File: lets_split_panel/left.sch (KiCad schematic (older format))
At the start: 69 parts, among them J1 Speaker, J2 RST, J3 ISP, P1 WS2812>, P2 USB_OTG, P3 >WS2812, P4 Conn_01x04, SW1 MXALPS, SW10 MXALPS, SW11 MXALPS, SW12 MXALPS, SW13 MXALPS, SW14 MXALPS, SW15 MXALPS, SW16 MXALPS, SW17 MXALPS, SW18 MXALPS, SW19 MXALPS, SW2 MXALPS, SW20 MXALPS, SW21 MXALPS, SW22 MXALPS, SW23 MXALPS, SW24 MXALPS, SW3 MXALPS, SW4 MXALPS, SW5 MXALPS, SW6 MXALPS, SW7 MXALPS, SW8 MXALPS, SW9 MXALPS, U1 ATMega32U4, Y1 Crystal

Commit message: I love git. Saved PCB file, started panel work
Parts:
- JP1, JP2: symbol JUMPER -> Jumper
- P1, P3: symbol CONN_01X03 -> Conn_01x03
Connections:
- net labels added: wd2812-in, ~Reset
- net labels removed: WD2812-in, ~RESET
- wire segments 132 -> 219

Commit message: Finished panel
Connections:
- net labels added: Dd+, Dd-
- wire segments 219 -> 154

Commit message: Added test jig for panel
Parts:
- removed P1: WS2812>, Wirepads:SMD_PAD_1x03_Pitch2.54mm, symbol Conn_01x03
- added J7: WS2812>, Pin_Headers:Pin_Header_Straight_1x01_Pitch2.54mm, symbol conn:Conn_01x01
- C1, C2, C3, C4: symbol C_Small -> lets_split_panel-rescue:C_Small-RESCUE-lets_split_panel
- D1, D10, D11, D12, D13, D14, D15, D16, D17, D18, D19, D2, D20, D21, D22, D23, D24, D3, D4, D5, D6, D7, D8, D9: symbol D -> lets_split_panel-rescue:D-RESCUE-lets_split_panel
- J1, J2: symbol Conn_01x02 -> lets_split_panel-rescue:Conn_01x02-RESCUE-lets_split_panel
- J3: footprint Jlink:J-link-needle-6pin -> Pin_Headers:Pin_Header_Straight_2x03_Pitch2.54mm; symbol Conn_02x03_Odd_Even -> lets_split_panel-rescue:Conn_02x03_Odd_Even-RESCUE-lets_split_panel
- JP1, JP2: symbol Jumper -> lets_split_panel-rescue:Jumper-RESCUE-lets_split_panel
- P2: symbol USB_OTG-RESCUE-lets_split -> lets_split_panel-rescue:USB_OTG-RESCUE-lets_split-RESCUE-lets_split_panel
- P3: symbol Conn_01x03 -> lets_split_panel-rescue:Conn_01x03-RESCUE-lets_split_panel
- P4: symbol Conn_01x04 -> lets_split_panel-rescue:Conn_01x04-RESCUE-lets_split_panel
- R1, R2, R3, R4, R5, R6: symbol R_Small -> lets_split_panel-rescue:R_Small-RESCUE-lets_split_panel
- SW1, SW10, SW11, SW12, SW13, SW14, SW15, SW16, SW17, SW18, SW19, SW2, SW20, SW21, SW22, SW23, SW24, SW3, SW4, SW5, SW6, SW7, SW8, SW9: symbol MXALPS -> lets_split_panel-rescue:MXALPS-RESCUE-lets_split_panel
- U1: symbol ATMega32U4 -> lets_split_panel-rescue:ATMega32U4-RESCUE-lets_split_panel
- Y1: symbol Crystal -> lets_split_panel-rescue:Crystal-RESCUE-lets_split_panel
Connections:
- wire segments 154 -> 150

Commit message: Changed to use SOT-23 dual diodes for cost
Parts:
- removed D1, D10, D11, D12, D13, D14, D15, D16, D17, D18, D19, D2, D20, D21, D22, D23, D24, D3, D4, D5, D6, D7, D8, D9: D, SeeedOPL-Diode-2016:SOD-123, symbol lets_split_panel-rescue:D-RESCUE-lets_split_panel
- removed SW1, SW10, SW11, SW12, SW13, SW14, SW15, SW16, SW17, SW18, SW19, SW2, SW20, SW21, SW22, SW23, SW24, SW3, SW4, SW5, SW6, SW7, SW8, SW9: MXALPS, CherryMX:Kailh-socket, symbol lets_split_panel-rescue:MXALPS-RESCUE-lets_split_panel
- added D1, D10, D11, D12, D2, D3, D4, D5, D6, D7, D8, D9: D_x2_KCom_AAK, TO_SOT_Packages_SMD:SOT-23, symbol device:D_x2_KCom_AAK
- added SW1, SW10, SW11, SW12, SW13, SW14, SW15, SW16, SW17, SW18, SW19, SW2, SW20, SW21, SW22, SW23, SW24, SW3, SW4, SW5, SW6, SW7, SW8, SW9: Socket, CherryMX:Kailh-socket, symbol switches:SW_Push
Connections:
- wire segments 150 -> 138
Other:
- moved on the sheet: P4

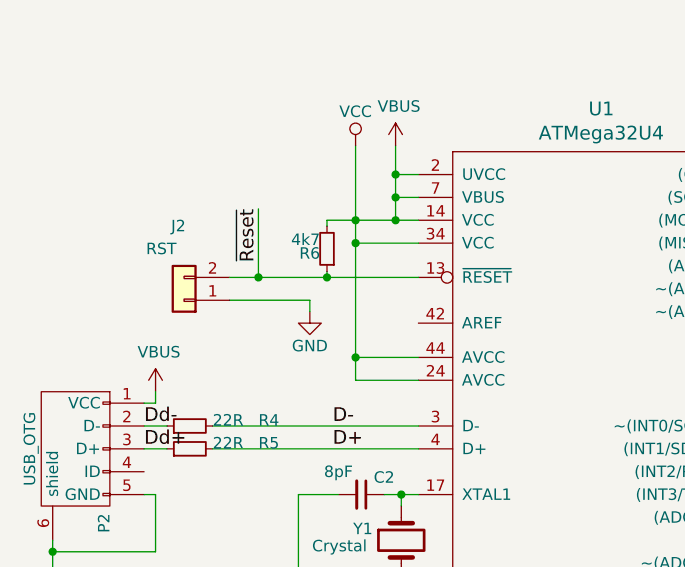
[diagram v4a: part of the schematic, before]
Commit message: Added fancy :)
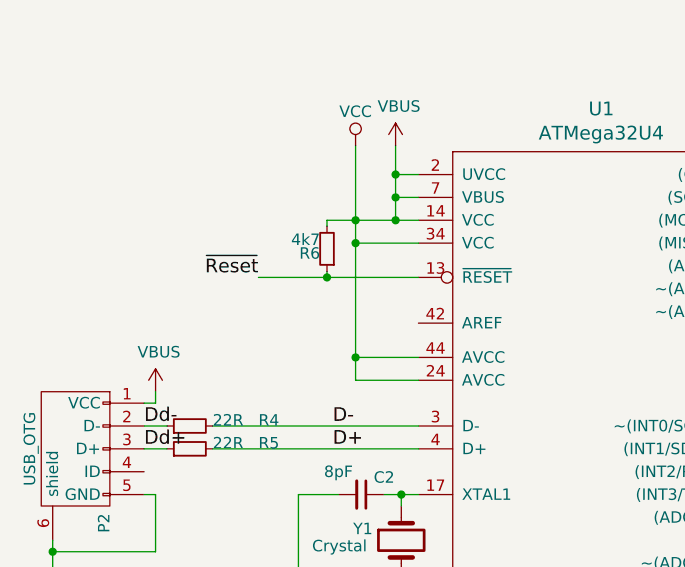
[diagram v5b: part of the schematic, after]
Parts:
- removed J2: RST, Pin_Headers:Pin_Header_Straight_1x02_Pitch2.54mm, symbol lets_split_panel-rescue:Conn_01x02-RESCUE-lets_split_panel
- C1, C4: footprint SeeedOPL-Capacitor-2016:C0603 -> Capacitors_SMD:C_0603
- C2, C3: footprint SeeedOPL-Capacitor-2016:C0402 -> Capacitors_SMD:C_0603
- R1, R2, R3, R4, R5, R6: footprint Resistors_SMD:R_0603_HandSoldering -> Resistors_SMD:R_0603
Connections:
- wire segments 138 -> 135
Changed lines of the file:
@@
 F 0 "R2" H 3530 2020 50  0000 L CNN
 F 1 "4k7" H 3530 1960 50  0000 L CNN
-F 2 "Resistors_SMD:R_0603_HandSoldering" H 3500 2000 50  0001 C CNN
+F 2 "Resistors_SMD:R_0603" H 3500 2000 50  0001 C CNN
 F 3 "" H 3500 2000 50  0000 C CNN
 	1    3500 2000
@@
 F 0 "R1" H 3430 2020 50  0000 L CNN
 F 1 "4k7" H 3430 1960 50  0000 L CNN
-F 2 "Resistors_SMD:R_0603_HandSoldering" H 3400 2000 50  0001 C CNN
+F 2 "Resistors_SMD:R_0603" H 3400 2000 50  0001 C CNN
 F 3 "" H 3400 2000 50  0000 C CNN
 	1    3400 2000
@@
 F 0 "R3" H 3305 3395 50  0000 L CNN
 F 1 "200" H 3305 3335 50  0000 L CNN
-F 2 "Resistors_SMD:R_0603_HandSoldering" H 3275 3375 50  0001 C CNN
+F 2 "Resistors_SMD:R_0603" H 3275 3375 50  0001 C CNN
 F 3 "" H 3275 3375 50  0000 C CNN
 	1    3275 3375
@@
 F 0 "R6" H 2230 4920 50  0000 L CNN
 F 1 "4k7" H 2230 4860 50  0000 L CNN
-F 2 "Resistors_SMD:R_0603_HandSoldering" H 2200 4900 50  0001 C CNN
+F 2 "Resistors_SMD:R_0603" H 2200 4900 50  0001 C CNN
 F 3 "" H 2200 4900 50  0000 C CNN
 	1    2200 4900
@@
 F 0 "C4" H 2542 6771 50  0000 L CNN
 F 1 "1uF" H 2542 6680 50  0000 L CNN
-F 2 "SeeedOPL-Capacitor-2016:C0603" H 2450 6725 50  0001 C CNN
+F 2 "Capacitors_SMD:C_0603" H 2450 6725 50  0001 C CNN
 F 3 "" H 2450 6725 50  0001 C CNN
 	1    2450 6725
@@
 F 0 "C2" V 2275 6075 50  0000 C CNN
 F 1 "8pF" V 2250 5875 50  0000 C CNN
-F 2 "SeeedOPL-Capacitor-2016:C0402" H 2350 5975 50  0001 C CNN
+F 2 "Capacitors_SMD:C_0603" H 2350 5975 50  0001 C CNN
 F 3 "" H 2350 5975 50  0001 C CNN
 	1    2350 5975
@@
 F 0 "C3" V 2525 6375 50  0000 C CNN
 F 1 "8pF" V 2450 6375 50  0000 C CNN
-F 2 "SeeedOPL-Capacitor-2016:C0402" H 2350 6375 50  0001 C CNN
+F 2 "Capacitors_SMD:C_0603" H 2350 6375 50  0001 C CNN
 F 3 "" H 2350 6375 50  0001 C CNN
 	1    2350 6375
@@
 F 0 "R4" V 1625 5375 50  0000 R CNN
 F 1 "22R" V 1625 5575 50  0000 R CNN
-F 2 "Resistors_SMD:R_0603_HandSoldering" H 1600 5675 50  0001 C CNN
+F 2 "Resistors_SMD:R_0603" H 1600 5675 50  0001 C CNN
 F 3 "" H 1600 5675 50  0000 C CNN
 	1    1600 5675
@@
 F 0 "R5" V 1625 5475 50  0000 R CNN
 F 1 "22R" V 1625 5675 50  0000 R CNN
-F 2 "Resistors_SMD:R_0603_HandSoldering" H 1600 5775 50  0001 C CNN
+F 2 "Resistors_SMD:R_0603" H 1600 5775 50  0001 C CNN
 F 3 "" H 1600 5775 50  0000 C CNN
 	1    1600 5775
@@
 F 0 "C1" H 2242 7321 50  0000 L CNN
 F 1 "1uF" H 2242 7230 50  0000 L CNN
-F 2 "SeeedOPL-Capacitor-2016:C0603" H 2150 7275 50  0001 C CNN
+F 2 "Capacitors_SMD:C_0603" H 2150 7275 50  0001 C CNN
 F 3 "" H 2150 7275 50  0001 C CNN
 	1    2150 7275
@@
 	-1   0    0    -1
 $EndComp
-$Comp
-L lets_split_panel-rescue:Conn_01x02-RESCUE-lets_split_panel J2
-U 1 1 5A0F48A9
-P 1575 5125
-F 0 "J2" H 1600 4800 50  0000 C CNN
-F 1 "RST" H 1675 4900 50  0000 C CNN
-F 2 "Pin_Headers:Pin_Header_Straight_1x02_Pitch2.54mm" H 1575 5125 50  0001 C CNN
-F 3 "" H 1575 5125 50  0001 C CNN
-	1    1575 5125
-	-1   0    0    1
-$EndComp
-$Comp
-L lets_split_panel-rescue:GND-RESCUE-lets_split_panel #PWR015
-U 1 1 5A0F501A
-P 2125 5175
-F 0 "#PWR015" H 2125 4925 50  0001 C CNN
-F 1 "GND" H 2125 5025 50  0000 C CNN
-F 2 "" H 2125 5175 50  0000 C CNN
-F 3 "" H 2125 5175 50  0000 C CNN
-	1    2125 5175
-	1    0    0    -1
-$EndComp
 Text Label 2225 5675 0    60   ~ 0
 D-
@@
 Wire Wire Line
 	6050 7050 6100 7050
-Connection ~ 1900 5025
-Wire Wire Line
-	1900 4725 1900 5025
 Connection ~ 3450 1225
 Wire Wire Line
@@
 Wire Wire Line
 	2600 6775 2550 6775
-Wire Wire Line
-	2125 5125 2125 5175
-Wire Wire Line
-	1775 5125 2125 5125
 Connection ~ 1000 6225
 Wire Wire Line
@@
 	2200 4775 2200 4800
 Connection ~ 2200 5025
-Wire Wire Line
-	1775 5025 2600 5025
 Wire Wire Line
 	2200 5025 2200 5000
@@
 Text Label 5500 7050 2    60   ~ 0
 ~Reset
-Text Label 1900 4725 3    60   ~ 0
+Text Label 1900 5025 2    60   ~ 0
 ~Reset
 Wire Wire Line
@@
 Connection ~ 10600 3525
 Connection ~ 10600 2875
+Wire Wire Line
+	1900 5025 2600 5025
 $EndSCHEMATC

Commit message: Seperated gerbers on request from board house
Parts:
- J7: symbol conn:Conn_01x01 -> lets_split_panel-rescue:Conn_01x01-RESCUE-lets_split_panel
- SW1, SW10, SW11, SW12, SW13, SW14, SW15, SW16, SW17, SW18, SW19, SW2, SW20, SW21, SW22, SW23, SW24, SW3, SW4, SW5, SW6, SW7, SW8, SW9: symbol switches:SW_Push -> lets_split_panel-rescue:SW_Push-RESCUE-lets_split_panel
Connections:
- wire segments 135 -> 182
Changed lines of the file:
@@
 	3500 1225 3500 1250
 Wire Wire Line
-	3400 1225 3500 1225
+	3400 1225 3450 1225
 Wire Wire Line
 	3400 1250 3400 1225
@@
 	1000 6225 1450 6225
 Wire Wire Line
-	2075 5975 2075 6450
+	2075 5975 2075 6375
 Wire Wire Line
 	2450 7275 2600 7275
@@
 	2075 5975 2250 5975
 Wire Wire Line
-	1000 6175 1000 6300
+	1000 6175 1000 6225
 Wire Wire Line
 	1450 5575 1450 5525
@@
 	2500 4675 2600 4675
 Wire Wire Line
-	2500 4775 2500 4450
+	2500 4775 2500 4675
 Wire Wire Line
 	2200 4775 2200 4800
@@
 	2200 5025 2200 5000
 Wire Wire Line
-	2450 6375 2600 6375
+	2450 6375 2525 6375
 Wire Wire Line
 	2525 6325 2525 6375
 Wire Wire Line
-	2450 5975 2600 5975
+	2450 5975 2525 5975
 Wire Wire Line
 	2525 6025 2525 5975
@@
 Connection ~ 2450 6975
 Wire Wire Line
-	2450 6875 2600 6875
+	2450 6875 2550 6875
 Connection ~ 2450 7075
 Wire Wire Line
@@
 	3400 2150 3400 2100
 Wire Wire Line
-	3075 2150 3825 2150
+	3075 2150 3400 2150
 Wire Wire Line
 	3500 2250 3500 2100
 Wire Wire Line
-	2950 2250 3950 2250
-Wire Wire Line
-	2325 4450 2325 5475
-Wire Wire Line
-	2200 4775 2600 4775
+	2950 2250 3500 2250
+Wire Wire Line
+	2325 4450 2325 4775
+Wire Wire Line
+	2200 4775 2325 4775
 Connection ~ 2450 7175
 Wire Wire Line
@@
 	2450 7175 2600 7175
 Wire Wire Line
-	2450 6825 2450 7375
+	2450 6825 2450 6875
 Wire Wire Line
 	4875 1375 5300 1375
@@
 Dd+
 $Comp
-L conn:Conn_01x01 J7
+L lets_split_panel-rescue:Conn_01x01-RESCUE-lets_split_panel J7
 U 1 1 5A14B17F
 P 3750 2775
@@
 $EndComp
 $Comp
-L switches:SW_Push SW1
+L lets_split_panel-rescue:SW_Push-RESCUE-lets_split_panel SW1
 U 1 1 5A172F2E
 P 6150 2875
@@
 	5950 2875 5900 2875
 Wire Wire Line
-	5900 2550 5900 4825
-Wire Wire Line
-	7400 2550 7400 4825
+	5900 2550 5900 2875
+Wire Wire Line
+	7400 2550 7400 2875
 Wire Wire Line
 	7400 2875 7350 2875
@@
 	6650 3075 6650 3125
 Wire Wire Line
-	5800 3125 9850 3125
+	5800 3125 6650 3125
 $Comp
 L device:D_x2_KCom_AAK D2
@@
 	7550 2875 7500 2875
 Wire Wire Line
-	7500 2550 7500 4825
-Wire Wire Line
-	9000 2550 9000 4825
+	7500 2550 7500 2875
+Wire Wire Line
+	9000 2550 9000 2875
 Wire Wire Line
 	9000 2875 8950 2875
@@
 	9150 2875 9100 2875
 Wire Wire Line
-	9100 2550 9100 4825
-Wire Wire Line
-	10600 2550 10600 4825
+	9100 2550 9100 2875
+Wire Wire Line
+	10600 2550 10600 2875
 Wire Wire Line
 	10600 2875 10550 2875
@@
 Connection ~ 8250 3125
 $Comp
-L switches:SW_Push SW2
+L lets_split_panel-rescue:SW_Push-RESCUE-lets_split_panel SW2
 U 1 1 5A176382
 P 7150 2875
@@
 $EndComp
 $Comp
-L switches:SW_Push SW3
+L lets_split_panel-rescue:SW_Push-RESCUE-lets_split_panel SW3
 U 1 1 5A1763EE
 P 7750 2875
@@
 $EndComp
 $Comp
-L switches:SW_Push SW4
+L lets_split_panel-rescue:SW_Push-RESCUE-lets_split_panel SW4
 U 1 1 5A176446
 P 8750 2875
@@
 $EndComp
 $Comp
-L switches:SW_Push SW5
+L lets_split_panel-rescue:SW_Push-RESCUE-lets_split_panel SW5
 U 1 1 5A1764A4
 P 9350 2875
@@
 $EndComp
 $Comp
-L switches:SW_Push SW6
+L lets_split_panel-rescue:SW_Push-RESCUE-lets_split_panel SW6
 U 1 1 5A1764FE
 P 10350 2875
@@
 $EndComp
 $Comp
-L switches:SW_Push SW7
+L lets_split_panel-rescue:SW_Push-RESCUE-lets_split_panel SW7
 U 1 1 5A1768AA
 P 6150 3525
@@
 	6650 3725 6650 3775
 Wire Wire Line
-	5800 3775 9850 3775
+	5800 3775 6650 3775
 $Comp
 L device:D_x2_KCom_AAK D5
@@
 Connection ~ 8250 3775
 $Comp
-L switches:SW_Push SW8
+L lets_split_panel-rescue:SW_Push-RESCUE-lets_split_panel SW8
 U 1 1 5A1768D3
 P 7150 3525
@@
 $EndComp
 $Comp
-L switches:SW_Push SW9
+L lets_split_panel-rescue:SW_Push-RESCUE-lets_split_panel SW9
 U 1 1 5A1768DA
 P 7750 3525
@@
 $EndComp
 $Comp
-L switches:SW_Push SW10
+L lets_split_panel-rescue:SW_Push-RESCUE-lets_split_panel SW10
 U 1 1 5A1768E1
 P 8750 3525
@@
 $EndComp
 $Comp
-L switches:SW_Push SW11
+L lets_split_panel-rescue:SW_Push-RESCUE-lets_split_panel SW11
 U 1 1 5A1768E8
 P 9350 3525
@@
 $EndComp
 $Comp
-L switches:SW_Push SW12
+L lets_split_panel-rescue:SW_Push-RESCUE-lets_split_panel SW12
 U 1 1 5A1768EF
 P 10350 3525
@@
 $EndComp
 $Comp
-L switches:SW_Push SW13
+L lets_split_panel-rescue:SW_Push-RESCUE-lets_split_panel SW13
 U 1 1 5A1773CA
 P 6150 4175
@@
 	6650 4375 6650 4425
 Wire Wire Line
-	5800 4425 9850 4425
+	5800 4425 6650 4425
 $Comp
 L device:D_x2_KCom_AAK D8
@@
 Connection ~ 8250 4425
 $Comp
-L switches:SW_Push SW14
+L lets_split_panel-rescue:SW_Push-RESCUE-lets_split_panel SW14
 U 1 1 5A1773F3
 P 7150 4175
@@
 $EndComp
 $Comp
-L switches:SW_Push SW15
+L lets_split_panel-rescue:SW_Push-RESCUE-lets_split_panel SW15
 U 1 1 5A1773FA
 P 7750 4175
@@
 $EndComp
 $Comp
-L switches:SW_Push SW16
+L lets_split_panel-rescue:SW_Push-RESCUE-lets_split_panel SW16
 U 1 1 5A177401
 P 8750 4175
@@
 $EndComp
 $Comp
-L switches:SW_Push SW17
+L lets_split_panel-rescue:SW_Push-RESCUE-lets_split_panel SW17
 U 1 1 5A177408
 P 9350 4175
@@
 $EndComp
 $Comp
-L switches:SW_Push SW18
+L lets_split_panel-rescue:SW_Push-RESCUE-lets_split_panel SW18
 U 1 1 5A17740F
 P 10350 4175
@@
 $EndComp
 $Comp
-L switches:SW_Push SW19
+L lets_split_panel-rescue:SW_Push-RESCUE-lets_split_panel SW19
 U 1 1 5A177699
 P 6150 4825
@@
 	6650 5025 6650 5075
 Wire Wire Line
-	5800 5075 9850 5075
+	5800 5075 6650 5075
 $Comp
 L device:D_x2_KCom_AAK D11
@@
 Connection ~ 8250 5075
 $Comp
-L switches:SW_Push SW20
+L lets_split_panel-rescue:SW_Push-RESCUE-lets_split_panel SW20
 U 1 1 5A1776C2
 P 7150 4825
@@
 $EndComp
 $Comp
-L switches:SW_Push SW21
+L lets_split_panel-rescue:SW_Push-RESCUE-lets_split_panel SW21
 U 1 1 5A1776C9
 P 7750 4825
@@
 $EndComp
 $Comp
-L switches:SW_Push SW22
+L lets_split_panel-rescue:SW_Push-RESCUE-lets_split_panel SW22
 U 1 1 5A1776D0
 P 8750 4825
@@
 $EndComp
 $Comp
-L switches:SW_Push SW23
+L lets_split_panel-rescue:SW_Push-RESCUE-lets_split_panel SW23
 U 1 1 5A1776D7
 P 9350 4825
@@
 $EndComp
 $Comp
-L switches:SW_Push SW24
+L lets_split_panel-rescue:SW_Push-RESCUE-lets_split_panel SW24
 U 1 1 5A1776DE
 P 10350 4825
@@
 Connection ~ 10600 2875
 Wire Wire Line
-	1900 5025 2600 5025
+	1900 5025 2200 5025
+Wire Wire Line
+	3450 1225 3500 1225
+Wire Wire Line
+	2500 4675 2500 4575
+Wire Wire Line
+	2500 4775 2600 4775
+Wire Wire Line
+	2550 6875 2600 6875
+Wire Wire Line
+	1000 6225 1000 6300
+Wire Wire Line
+	2075 6375 2075 6450
+Wire Wire Line
+	2525 5975 2600 5975
+Wire Wire Line
+	2525 6375 2600 6375
+Wire Wire Line
+	2450 6875 2450 6975
+Wire Wire Line
+	2500 4575 2500 4450
+Wire Wire Line
+	2200 5025 2600 5025
+Wire Wire Line
+	2325 5375 2325 5475
+Wire Wire Line
+	2325 4875 2325 5375
+Wire Wire Line
+	2325 4775 2325 4875
+Wire Wire Line
+	2325 4775 2500 4775
+Wire Wire Line
+	2450 6975 2450 7075
+Wire Wire Line
+	2450 7075 2450 7175
+Wire Wire Line
+	3500 2250 3950 2250
+Wire Wire Line
+	3400 2150 3825 2150
+Wire Wire Line
+	2450 7175 2450 7275
+Wire Wire Line
+	2450 7275 2450 7375
+Wire Wire Line
+	6650 3125 8250 3125
+Wire Wire Line
+	8250 3125 9850 3125
+Wire Wire Line
+	6650 3775 8250 3775
+Wire Wire Line
+	8250 3775 9850 3775
+Wire Wire Line
+	6650 4425 8250 4425
+Wire Wire Line
+	8250 4425 9850 4425
+Wire Wire Line
+	6650 5075 8250 5075
+Wire Wire Line
+	8250 5075 9850 5075
+Wire Wire Line
+	5900 4175 5900 4825
+Wire Wire Line
+	5900 3525 5900 4175
+Wire Wire Line
+	5900 2875 5900 3525
+Wire Wire Line
+	7400 2875 7400 3525
+Wire Wire Line
+	7500 2875 7500 3525
+Wire Wire Line
+	7400 3525 7400 4175
+Wire Wire Line
+	7500 3525 7500 4175
+Wire Wire Line
+	7400 4175 7400 4825
+Wire Wire Line
+	7500 4175 7500 4825
+Wire Wire Line
+	9000 2875 9000 3525
+Wire Wire Line
+	9000 3525 9000 4175
+Wire Wire Line
+	9000 4175 9000 4825
+Wire Wire Line
+	9100 4175 9100 4825
+Wire Wire Line
+	9100 3525 9100 4175
+Wire Wire Line
+	9100 2875 9100 3525
+Wire Wire Line
+	10600 4175 10600 4825
+Wire Wire Line
+	10600 3525 10600 4175
+Wire Wire Line
+	10600 2875 10600 3525
 $EndSCHEMATC

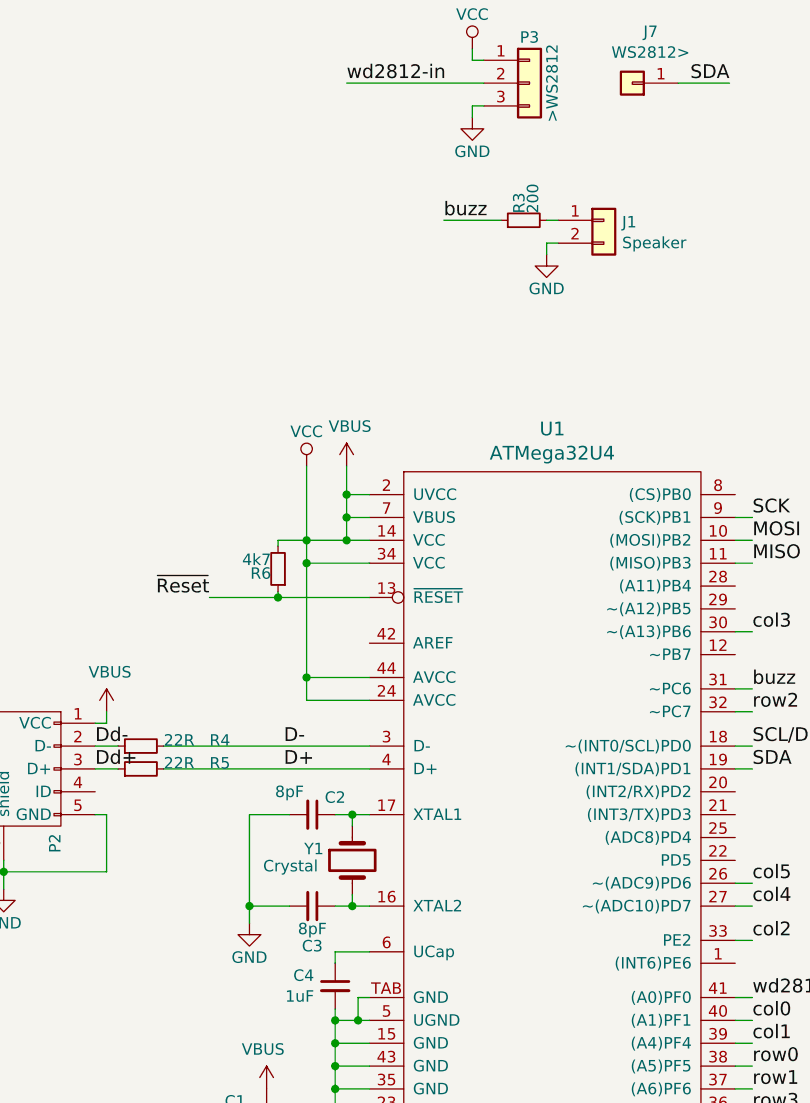
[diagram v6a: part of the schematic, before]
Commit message: Added PnP files and split gerbers
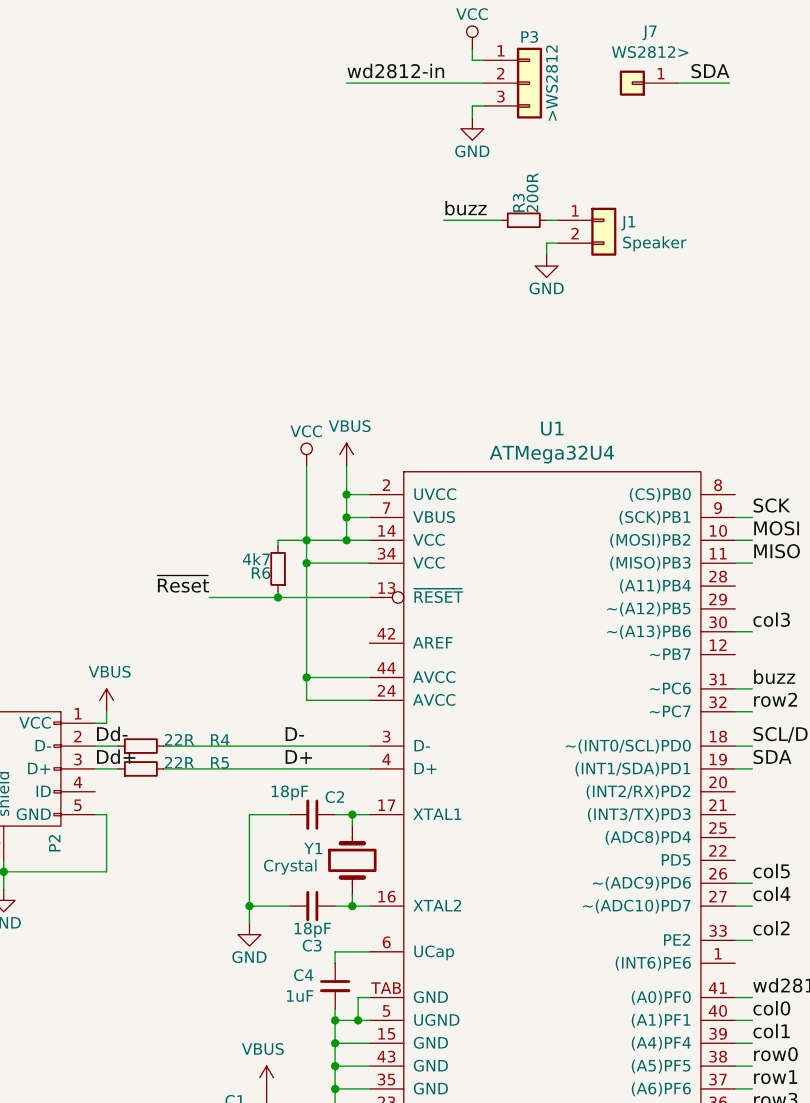
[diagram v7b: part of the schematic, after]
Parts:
- C2, C3: value 8pF -> 18pF
- R3: value 200 -> 200R
- Y1: footprint SeeedOPL-Crystal Oscillator-2016:X2-SMD-3.2X1.5X0.55MM -> Crystals:Crystal_SMD_Abracon_ABM3-2pin_5.0x3.2mm
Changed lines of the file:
@@
 P 3275 3375
 F 0 "R3" H 3305 3395 50  0000 L CNN
-F 1 "200" H 3305 3335 50  0000 L CNN
+F 1 "200R" H 3305 3335 50  0000 L CNN
 F 2 "Resistors_SMD:R_0603" H 3275 3375 50  0001 C CNN
 F 3 "" H 3275 3375 50  0000 C CNN
@@
 F 0 "Y1" V 2475 6300 50  0000 L CNN
 F 1 "Crystal" V 2550 6325 50  0000 L CNN
-F 2 "SeeedOPL-Crystal Oscillator-2016:X2-SMD-3.2X1.5X0.55MM" H 2525 6175 50  0001 C CNN
+F 2 "Crystals:Crystal_SMD_Abracon_ABM3-2pin_5.0x3.2mm" H 2525 6175 50  0001 C CNN
 F 3 "" H 2525 6175 50  0001 C CNN
 	1    2525 6175
@@
 P 2350 5975
 F 0 "C2" V 2275 6075 50  0000 C CNN
-F 1 "8pF" V 2250 5875 50  0000 C CNN
+F 1 "18pF" V 2250 5875 50  0000 C CNN
 F 2 "Capacitors_SMD:C_0603" H 2350 5975 50  0001 C CNN
 F 3 "" H 2350 5975 50  0001 C CNN
@@
 P 2350 6375
 F 0 "C3" V 2525 6375 50  0000 C CNN
-F 1 "8pF" V 2450 6375 50  0000 C CNN
+F 1 "18pF" V 2450 6375 50  0000 C CNN
 F 2 "Capacitors_SMD:C_0603" H 2350 6375 50  0001 C CNN
 F 3 "" H 2350 6375 50  0001 C CNN
